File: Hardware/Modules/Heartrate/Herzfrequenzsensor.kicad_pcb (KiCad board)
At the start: 2 copper layers, 35 x 35 mm, 12 parts, among them U1 MAX30101EFD_T, U2 TLV70018_SOT23-5, U4 PCA9306DCTR

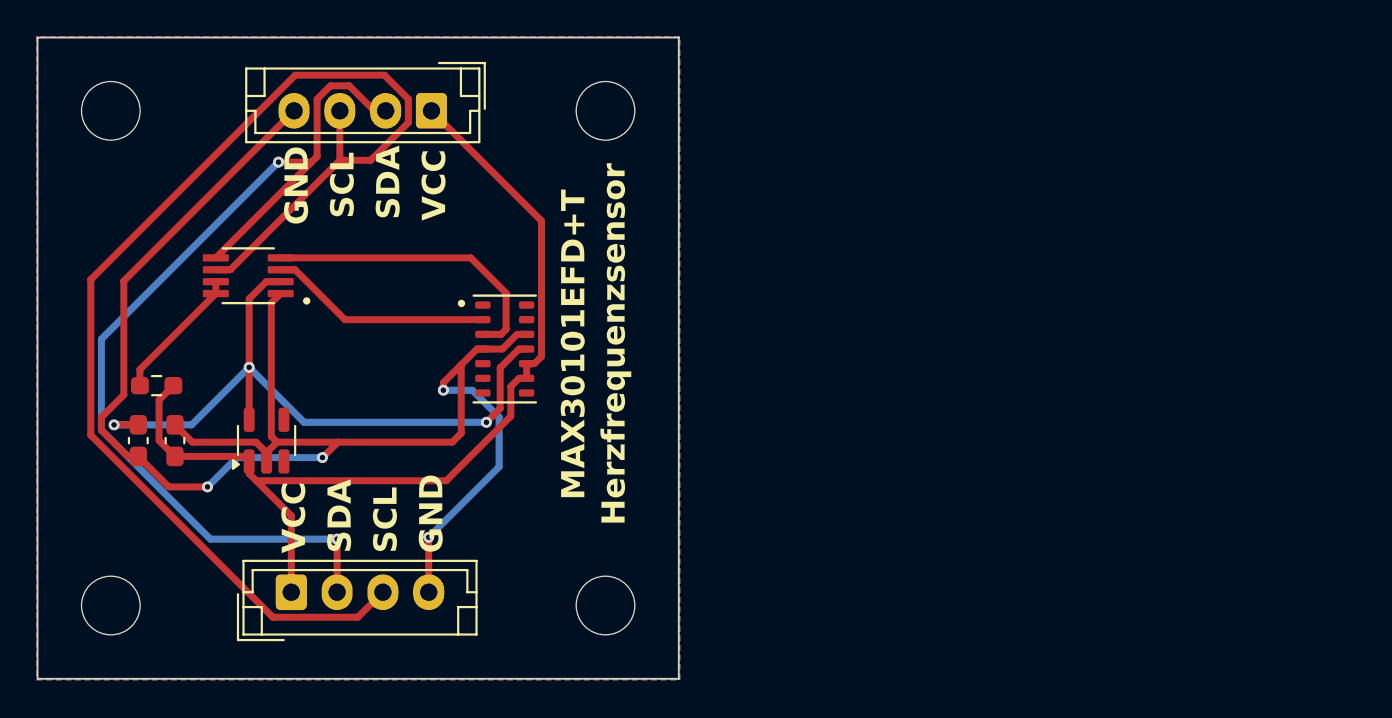
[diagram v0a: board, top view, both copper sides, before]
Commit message: HeartRateV2
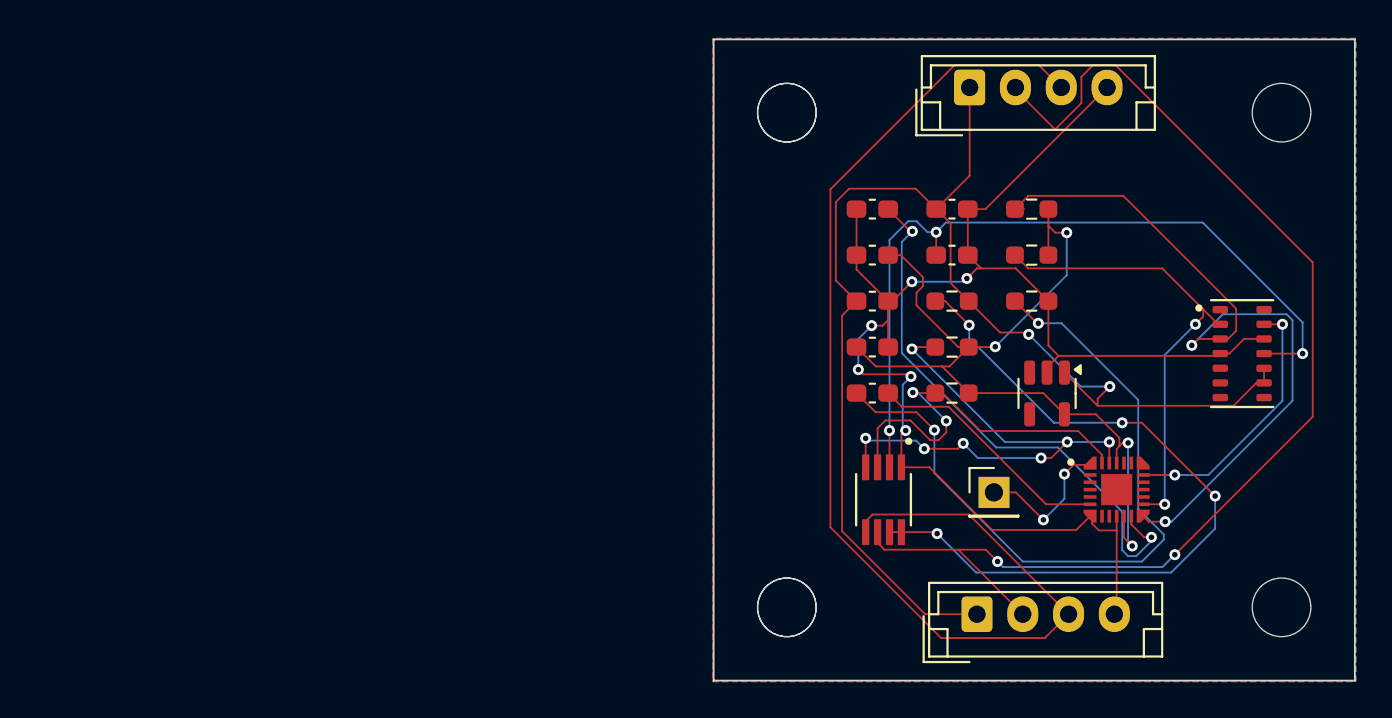
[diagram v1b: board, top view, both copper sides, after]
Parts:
- removed C3, C4: 1µ, Capacitor_SMD:C_0603_1608Metric_Pad1.08x0.95mm_HandSolder
- removed J1, J2: ~, Connector_JST:JST_EH_B4B-EH-A_1x04_P2.50mm_Vertical
- removed R1: 200k, Resistor_SMD:R_0603_1608Metric_Pad0.98x0.95mm_HandSolder
- removed the REF** at (113.2, 49.5)
- removed the REF** at (113.2, 76.5)
- removed the REF** at (86.2, 76.5)
- removed the REF** at (86.2, 49.5)
- removed U1: MAX30101EFD_T, Modular_Electronics_Toolkit:PSON80P560X330X165-14N
- removed U2: TLV70018_SOT23-5, Package_TO_SOT_SMD:SOT-23-5
- removed U4: PCA9306DCTR, Modular_Electronics_Toolkit:SOP65P400X130-8N
- added ?: , , F.Cu at (123.1, 76.6)
- added ?: , , F.Cu at (123.1, 49.6)
- added C10: 0.1µF, Capacitor_SMD:C_0603_1608Metric_Pad1.08x0.95mm_HandSolder, F.Cu at (127.8, 64.9)
- added C11: 4.7µF, Capacitor_SMD:C_0603_1608Metric_Pad1.08x0.95mm_HandSolder, F.Cu at (132.1, 54.9)
- added C12: 4.7µF, Capacitor_SMD:C_0603_1608Metric_Pad1.08x0.95mm_HandSolder, F.Cu at (132.1, 57.4)
- added C6: 1µ, Capacitor_SMD:C_0603_1608Metric_Pad1.08x0.95mm_HandSolder, F.Cu at (127.8, 54.9)
- added C7: 1µ, Capacitor_SMD:C_0603_1608Metric_Pad1.08x0.95mm_HandSolder, F.Cu at (127.8, 57.4)
- added C8: 1µ, Capacitor_SMD:C_0603_1608Metric_Pad1.08x0.95mm_HandSolder, F.Cu at (127.8, 59.9)
- added C9: 1µ, Capacitor_SMD:C_0603_1608Metric_Pad1.08x0.95mm_HandSolder, F.Cu at (127.8, 62.4)
- added J4: B4B-EH-A, Connector_JST:JST_EH_B4B-EH-A_1x04_P2.50mm_Vertical, F.Cu at (133.1, 48.2)
- added J5: B4B-EH-A, Connector_JST:JST_EH_B4B-EH-A_1x04_P2.50mm_Vertical, F.Cu at (133.5, 77.0)
- added J6: Conn_01x01_Pin, Connector_PinHeader_2.54mm:PinHeader_1x01_P2.54mm_Vertical, F.Cu at (134.4, 70.3)
- added R3: 200k, Resistor_SMD:R_0603_1608Metric_Pad0.98x0.95mm_HandSolder, F.Cu at (132.1, 59.9)
- added R4: 4.7k, Resistor_SMD:R_0603_1608Metric_Pad0.98x0.95mm_HandSolder, F.Cu at (132.1, 62.4)
- added R5: 4.7k, Resistor_SMD:R_0603_1608Metric_Pad0.98x0.95mm_HandSolder, F.Cu at (132.1, 64.9)
- added R6: 4.7k, Resistor_SMD:R_0603_1608Metric_Pad0.98x0.95mm_HandSolder, F.Cu at (136.5, 54.9)
- added R7: 4.7k, Resistor_SMD:R_0603_1608Metric_Pad0.98x0.95mm_HandSolder, F.Cu at (136.5, 57.4)
- added R8: 10R, Resistor_SMD:R_0603_1608Metric_Pad0.98x0.95mm_HandSolder, F.Cu at (136.5, 59.9)
- added REF**: MountingHole_3.2mm_M3, MountingHole:MountingHole_3.2mm_M3, F.Cu at (150.1, 49.6)
- added REF**: MountingHole_3.2mm_M3, MountingHole:MountingHole_3.2mm_M3, F.Cu at (123.1, 49.6)
- added REF**: MountingHole_3.2mm_M3, MountingHole:MountingHole_3.2mm_M3, F.Cu at (123.1, 76.6)
- added REF**: MountingHole_3.2mm_M3, MountingHole:MountingHole_3.2mm_M3, F.Cu at (150.1, 76.6)
- added U6: MAX30101EFD_T, Modular_Electronics_Toolkit:PSON80P560X330X165-14N, F.Cu at (148.0, 62.8)
- added U7: PCA9306DCTR, Modular_Electronics_Toolkit:SOP65P400X130-8N, F.Cu at (128.4, 70.7)
- added U8: MAX32664GTGA_T, Modular_Electronics_Toolkit:IC_MAX32664GTGA_T, F.Cu at (141.1, 70.2)
- added U9: TLV70018_SOT23-5, Package_TO_SOT_SMD:SOT-23-5, F.Cu at (137.3, 64.9)
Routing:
- net GND: track 87.2 -> 0.00 mm, vias 4 -> 0
- net VCORE: track 0.00 -> 81.0 mm, vias 0 -> 6
- net VCC: track 0.00 -> 71.3 mm, vias 0 -> 2
- net Net-(U4-SCL2): track 69.4 -> 0.00 mm
- net SCL: track 0.00 -> 65.7 mm, vias 0 -> 2
- net SDA: track 0.00 -> 64.5 mm
- net Net-(U4-SDA2): track 54.2 -> 0.00 mm, vias 2 -> 0
- net Net-(U1-VLED+): track 52.5 -> 0.00 mm
- net V18: track 0.00 -> 48.7 mm, vias 0 -> 4
- net VREF: track 0.00 -> 43.2 mm, vias 0 -> 3
- net Net-(U7-EN): track 0.00 -> 41.6 mm, vias 0 -> 4
- net B3: track 0.00 -> 41.3 mm, vias 0 -> 2
- net Net-(C10-Pad1): track 0.00 -> 39.6 mm, vias 0 -> 2
- net Net-(U1-VDD): track 38.1 -> 0.00 mm, vias 3 -> 0
- net Net-(U8-VCORE): track 0.00 -> 30.5 mm, vias 0 -> 2
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- added copper zone on F.Cu, net VCC
- added copper zone on B.Cu, net VCORE
- removed copper zone on F.Cu, net (none)
- removed copper zone on B.Cu, net GND
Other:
- board text removed: "GND"
- board text removed: "Herzfrequenzsensor"
- board text removed: "MAX30101EFD+T"
- board text removed: "SCL"
- board text removed: "SDA"
- board text removed: "VCC"
